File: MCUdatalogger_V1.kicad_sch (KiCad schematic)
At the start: 25 parts, among them U1 24LC1025, U2 DS1337S+, U3 24LC1025, U4 ATMEGA328P-AU, Y1 32.768 KHz, Y2 16 MHz

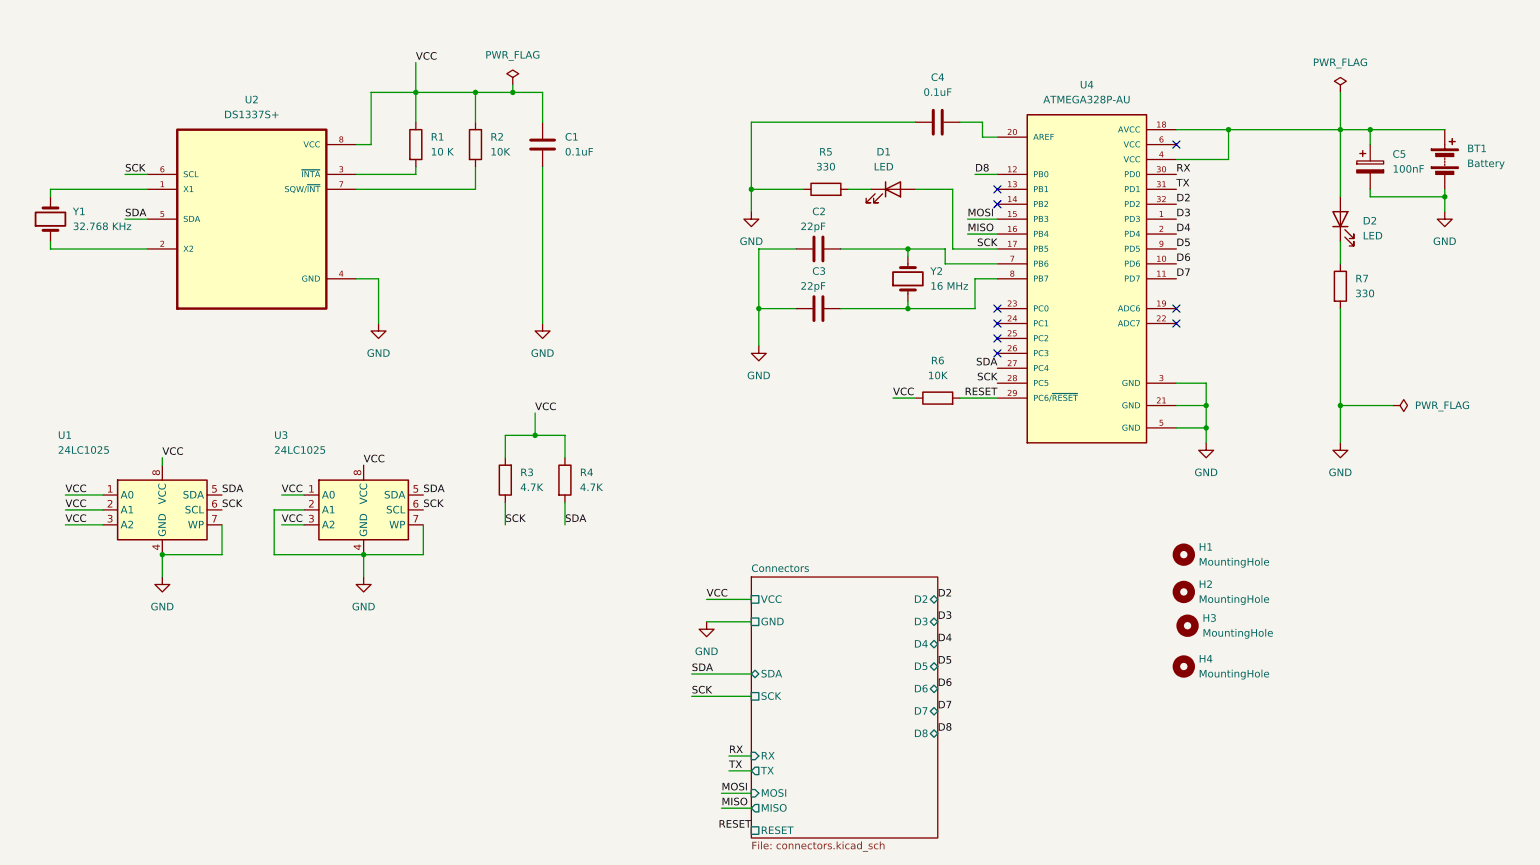
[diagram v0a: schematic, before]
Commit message: Completed comments.
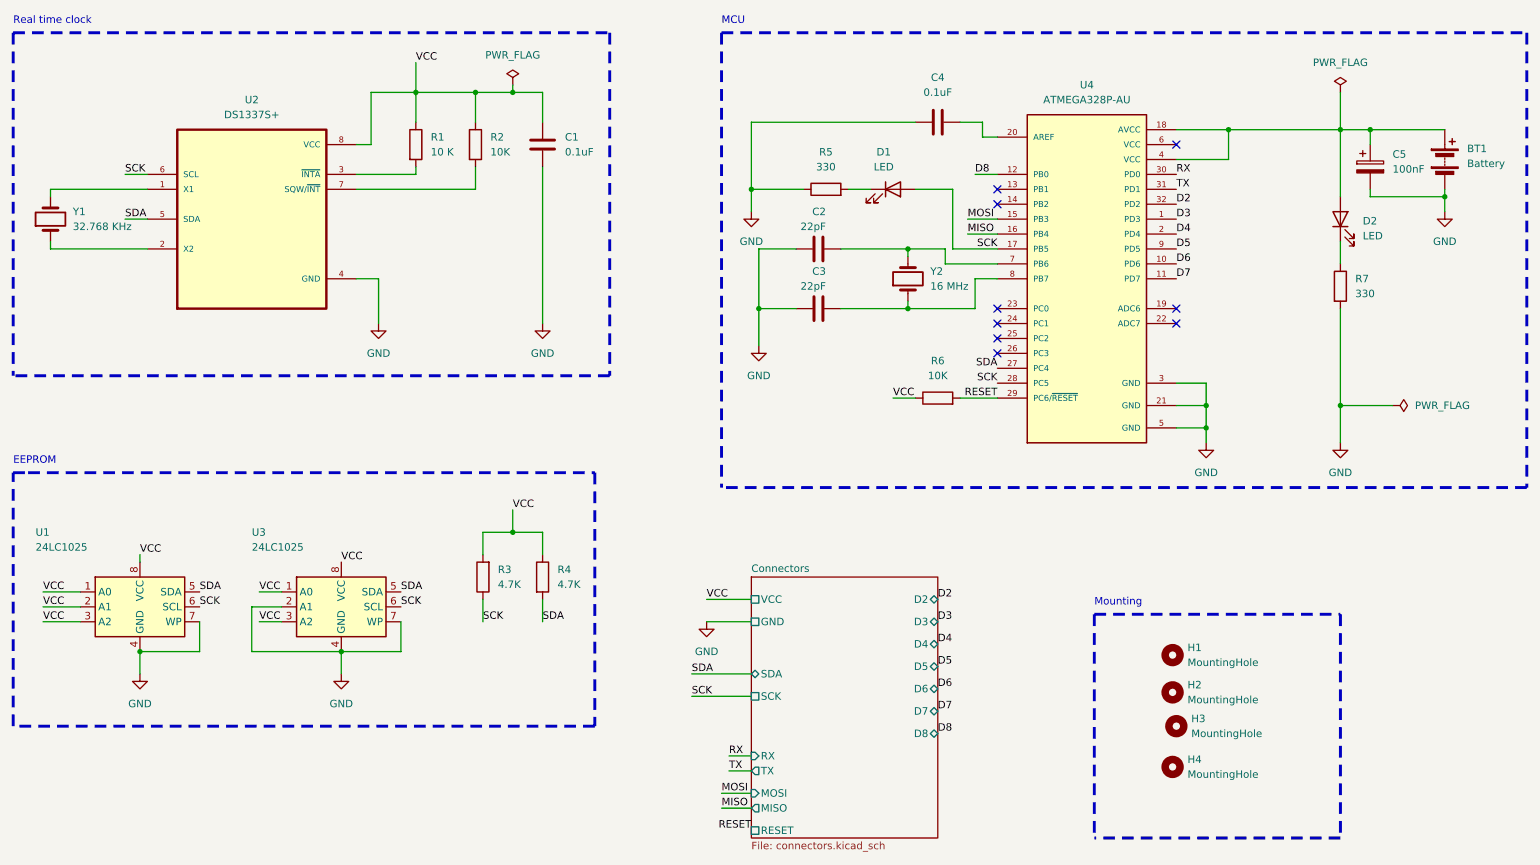
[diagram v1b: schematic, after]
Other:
- note added: "EEPROM"
- note added: "MCU"
- note added: "Mounting"
- note added: "Real time clock"
- moved on the sheet: H1, H2, H3, H4, R3, R4, U1, U3
